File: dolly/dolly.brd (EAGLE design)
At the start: 104.1 x 120.6 mm, 31 parts, among them U1 ATTINY85-20P

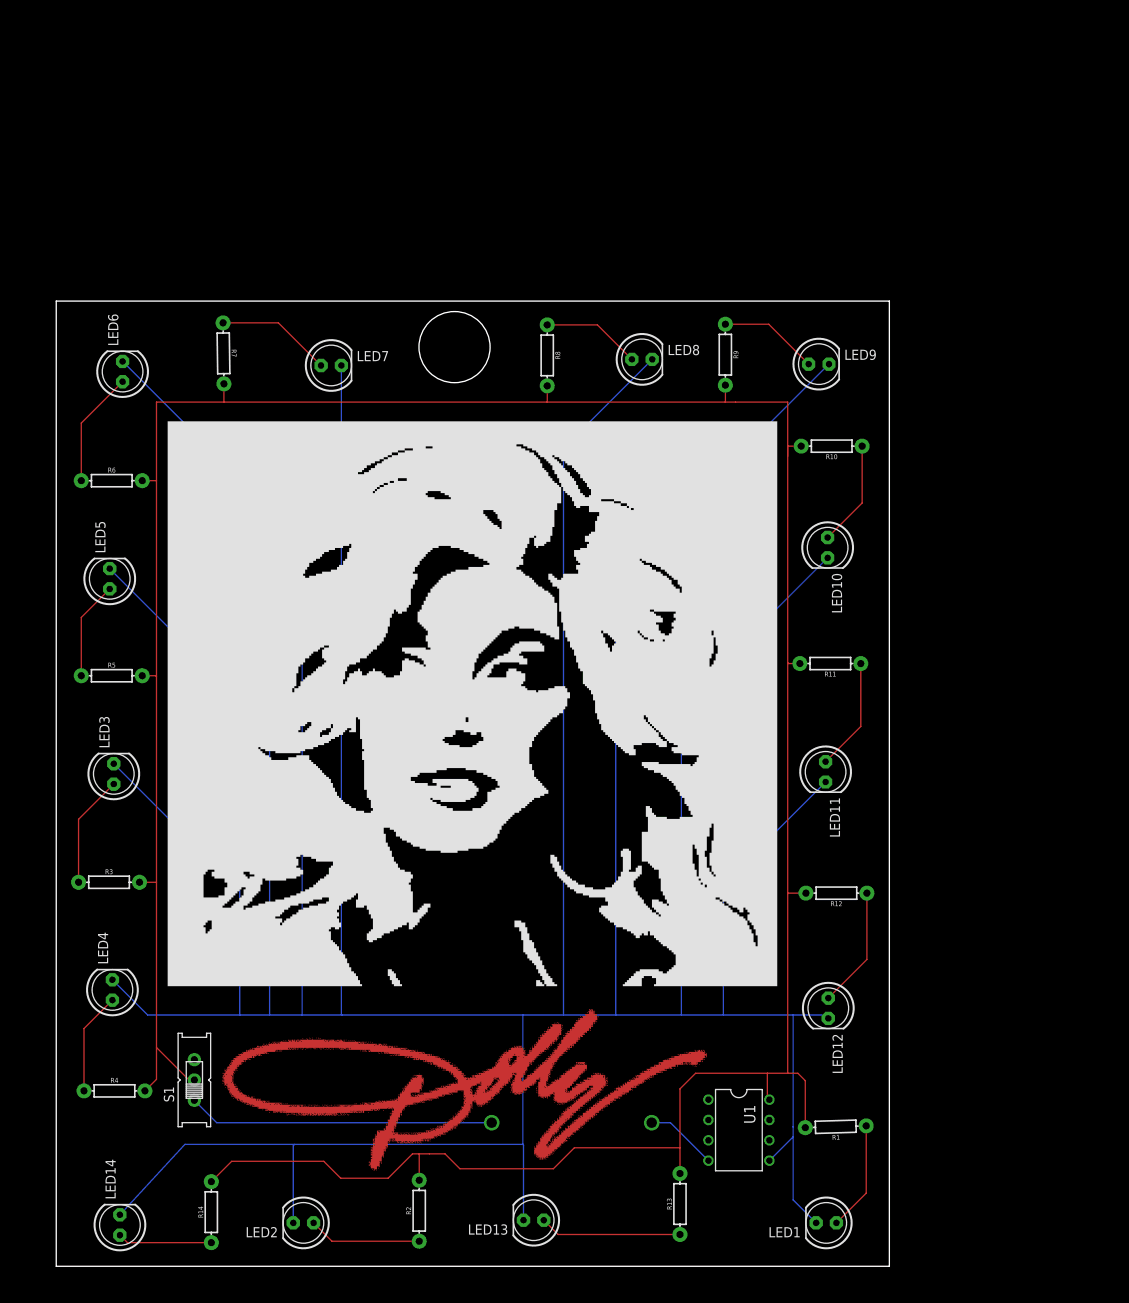
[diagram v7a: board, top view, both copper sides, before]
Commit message: resize dolly badge
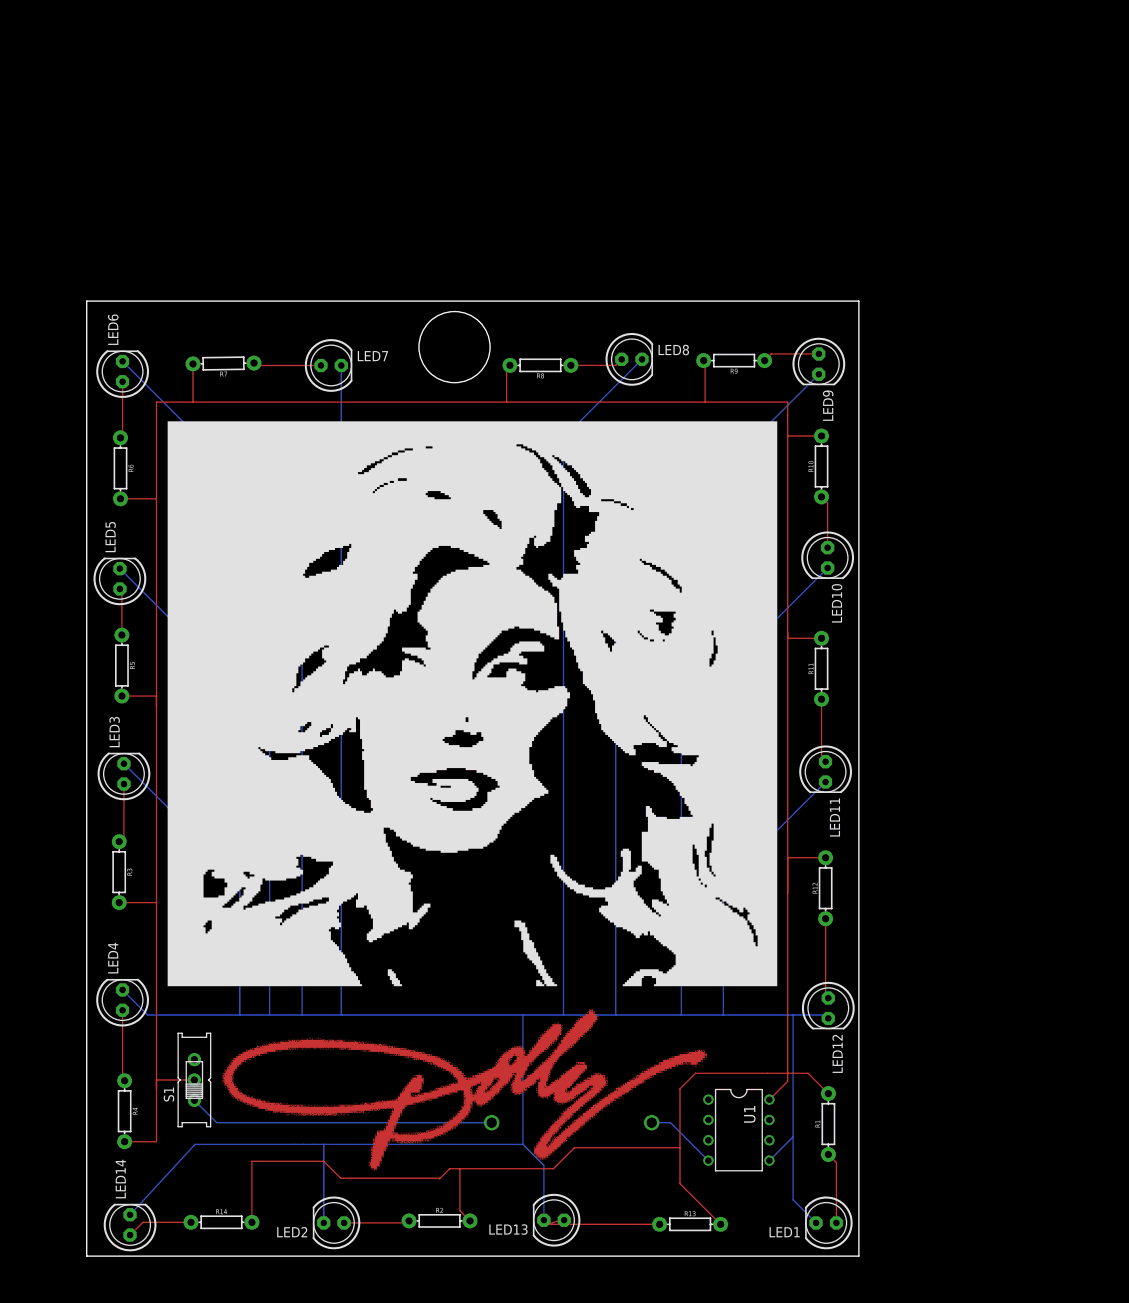
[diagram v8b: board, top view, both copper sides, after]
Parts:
- moved LED2 3.81 mm to (20.7, -4.74)
- moved R2 2.84 mm to (33.9, -4.49), turned to 0 degrees
- moved R13 2.84 mm to (65.3, -4.92), turned to 0 degrees
- moved R4 2.84 mm to (-5.42, 9.23), turned to 270 degrees
- moved R10 2.84 mm to (81.7, 89.8), turned to 90 degrees
- moved LED13 2.54 mm to (48.3, -4.40)
- moved R6 1.89 mm to (-5.94, 89.6), turned to 270 degrees
- moved R3 1.80 mm to (-6.10, 39.1), turned to 270 degrees
- moved LED4 1.80 mm to (-5.68, 23.1)
- moved R14 1.80 mm to (6.68, -4.66), turned to 0 degrees
- moved R5 1.80 mm to (-5.76, 64.9), turned to 270 degrees
- moved R8 1.51 mm to (46.6, 102.5), turned to 180 degrees
- moved R12 1.48 mm to (82.2, 37.1), turned to 90 degrees
- moved R9 1.32 mm to (70.8, 103.1), turned to 180 degrees
- moved R11 1.28 mm to (81.7, 64.5), turned to 90 degrees
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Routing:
- net N$6: track 378.6 -> 427.6 mm
- net N$9: track 14.5 -> 7.13 mm
- net N$4: track 765.0 -> 758.2 mm
- net N$13: track 13.2 -> 6.66 mm
- net N$8: track 12.3 -> 5.87 mm
- net N$3: track 14.1 -> 7.80 mm
- net N$14: track 14.1 -> 8.01 mm
- net N$10: track 14.5 -> 8.51 mm
- net N$18: track 14.2 -> 8.23 mm
- net N$11: track 12.4 -> 6.66 mm
- net N$12: track 12.5 -> 7.12 mm
- net N$15: track 15.1 -> 10.3 mm
- net N$1: track 13.7 -> 8.96 mm
- net N$7: track 12.8 -> 9.06 mm
- net N$17: track 11.8 -> 8.28 mm
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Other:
- board size 104.1 x 120.6 mm -> 96.5 x 119.4 mm
